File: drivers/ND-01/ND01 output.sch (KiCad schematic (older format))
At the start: 13 parts, among them J10 CONN_01X08, J11 CONN_01X08, J12 CONN_01X08, J13 CONN_01X08, J14 CONN_01X08, J15 CONN_01X08, J16 CONN_01X08, J4 CONN_01X08, J5 CONN_01X08, J6 CONN_01X08, J7 CONN_01X08, J8 CONN_01X08, J9 CONN_01X08

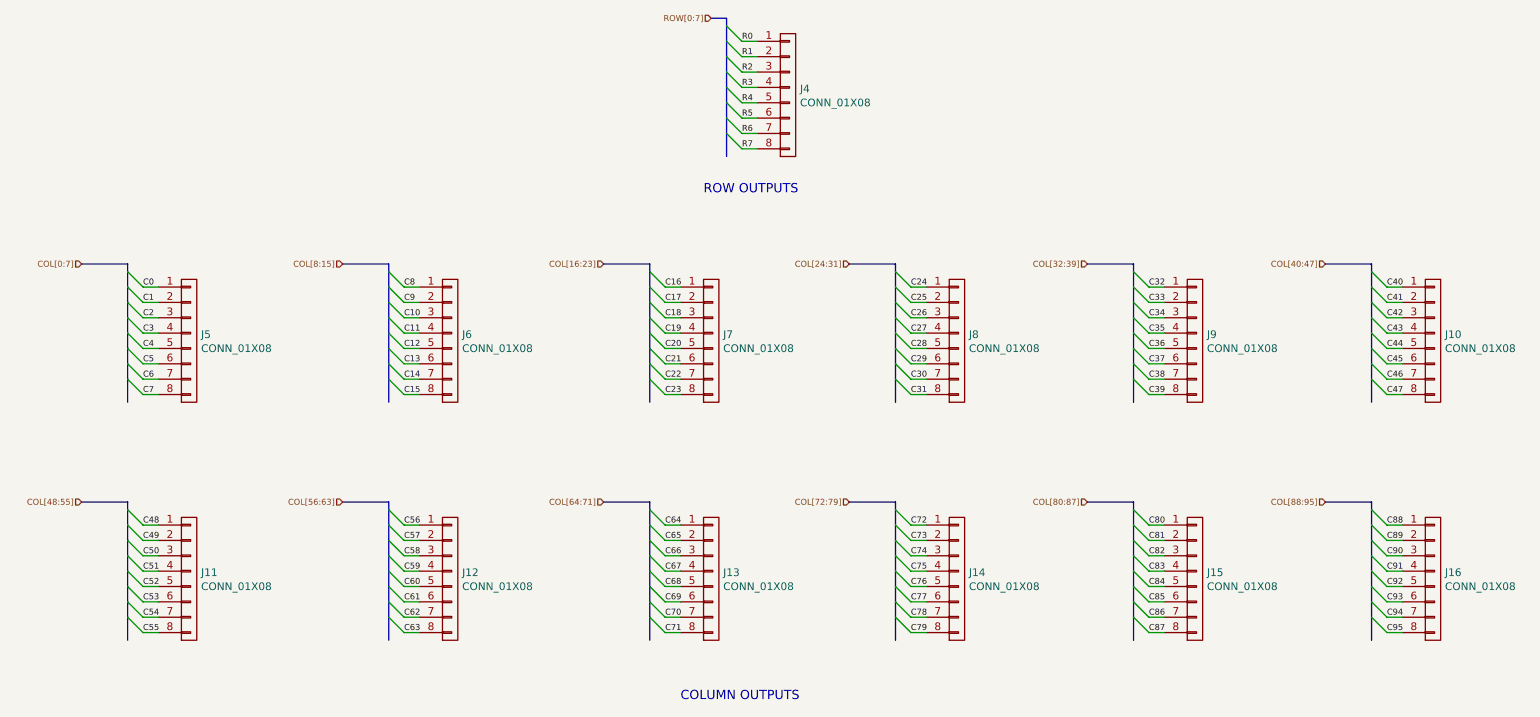
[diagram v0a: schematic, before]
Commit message: Add 2088xS LED dot matrix documentation pictures
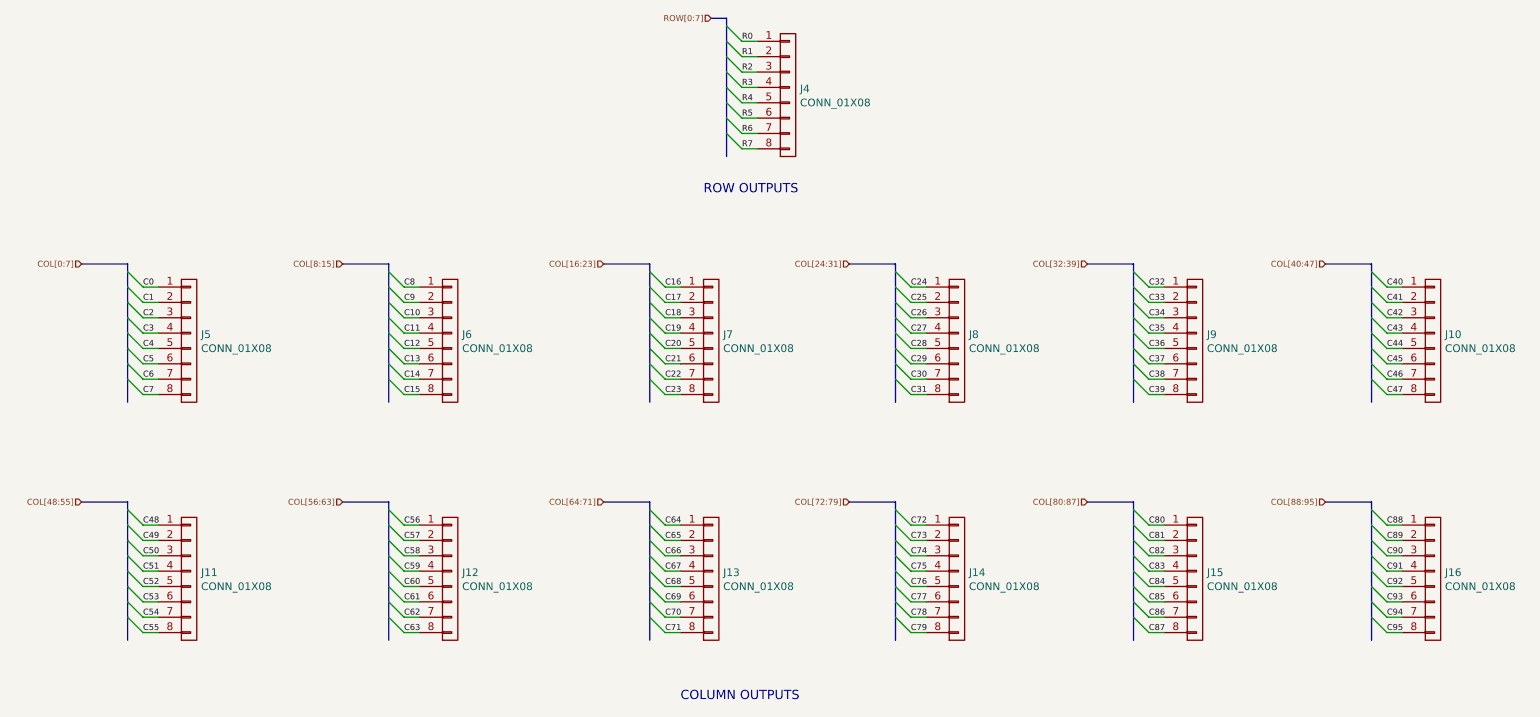
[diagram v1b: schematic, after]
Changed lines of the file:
@@
 	5300 900  5400 900
 Wire Bus Line
-	5400 900  5400 950
-Wire Bus Line
-	5400 950  5400 1050
-Wire Bus Line
-	5400 1050 5400 1150
-Wire Bus Line
-	5400 1150 5400 1250
-Wire Bus Line
-	5400 1250 5400 1350
-Wire Bus Line
-	5400 1350 5400 1450
-Wire Bus Line
-	5400 1450 5400 1550
-Wire Bus Line
-	5400 1550 5400 1650
-Wire Bus Line
-	5400 1650 5400 1800
+	5400 900  5400 1800
 $Comp
 L CONN_01X08 J4
@@
 	1200 2500 1500 2500
 Wire Bus Line
-	1500 2500 1500 2550
-Wire Bus Line
-	1500 2550 1500 2650
-Wire Bus Line
-	1500 2650 1500 2750
-Wire Bus Line
-	1500 2750 1500 2850
-Wire Bus Line
-	1500 2850 1500 2950
-Wire Bus Line
-	1500 2950 1500 3050
-Wire Bus Line
-	1500 3050 1500 3150
-Wire Bus Line
-	1500 3150 1500 3250
-Wire Bus Line
-	1500 3250 1500 3400
+	1500 2500 1500 3400
 $Comp
 L CONN_01X08 J5
@@
 	2900 2500 3200 2500
 Wire Bus Line
-	3200 2500 3200 2550
-Wire Bus Line
-	3200 2550 3200 2650
-Wire Bus Line
-	3200 2650 3200 2750
-Wire Bus Line
-	3200 2750 3200 2850
-Wire Bus Line
-	3200 2850 3200 2950
-Wire Bus Line
-	3200 2950 3200 3050
-Wire Bus Line
-	3200 3050 3200 3150
-Wire Bus Line
-	3200 3150 3200 3250
-Wire Bus Line
-	3200 3250 3200 3400
+	3200 2500 3200 3400
 $Comp
 L CONN_01X08 J6
@@
 	4600 2500 4900 2500
 Wire Bus Line
-	4900 2500 4900 2550
-Wire Bus Line
-	4900 2550 4900 2650
-Wire Bus Line
-	4900 2650 4900 2750
-Wire Bus Line
-	4900 2750 4900 2850
-Wire Bus Line
-	4900 2850 4900 2950
-Wire Bus Line
-	4900 2950 4900 3050
-Wire Bus Line
-	4900 3050 4900 3150
-Wire Bus Line
-	4900 3150 4900 3250
-Wire Bus Line
-	4900 3250 4900 3400
+	4900 2500 4900 3400
 $Comp
 L CONN_01X08 J7
@@
 	6200 2500 6500 2500
 Wire Bus Line
-	6500 2500 6500 2550
-Wire Bus Line
-	6500 2550 6500 2650
-Wire Bus Line
-	6500 2650 6500 2750
-Wire Bus Line
-	6500 2750 6500 2850
-Wire Bus Line
-	6500 2850 6500 2950
-Wire Bus Line
-	6500 2950 6500 3050
-Wire Bus Line
-	6500 3050 6500 3150
-Wire Bus Line
-	6500 3150 6500 3250
-Wire Bus Line
-	6500 3250 6500 3400
+	6500 2500 6500 3400
 $Comp
 L CONN_01X08 J8
@@
 	7750 2500 8050 2500
 Wire Bus Line
-	8050 2500 8050 2550
-Wire Bus Line
-	8050 2550 8050 2650
-Wire Bus Line
-	8050 2650 8050 2750
-Wire Bus Line
-	8050 2750 8050 2850
-Wire Bus Line
-	8050 2850 8050 2950
-Wire Bus Line
-	8050 2950 8050 3050
-Wire Bus Line
-	8050 3050 8050 3150
-Wire Bus Line
-	8050 3150 8050 3250
-Wire Bus Line
-	8050 3250 8050 3400
+	8050 2500 8050 3400
 $Comp
 L CONN_01X08 J9
@@
 	9300 2500 9600 2500
 Wire Bus Line
-	9600 2500 9600 2550
-Wire Bus Line
-	9600 2550 9600 2650
-Wire Bus Line
-	9600 2650 9600 2750
-Wire Bus Line
-	9600 2750 9600 2850
-Wire Bus Line
-	9600 2850 9600 2950
-Wire Bus Line
-	9600 2950 9600 3050
-Wire Bus Line
-	9600 3050 9600 3150
-Wire Bus Line
-	9600 3150 9600 3250
-Wire Bus Line
-	9600 3250 9600 3400
+	9600 2500 9600 3400
 $Comp
 L CONN_01X08 J10
@@
 	1200 4050 1500 4050
 Wire Bus Line
-	1500 4050 1500 4100
-Wire Bus Line
-	1500 4100 1500 4200
-Wire Bus Line
-	1500 4200 1500 4300
-Wire Bus Line
-	1500 4300 1500 4400
-Wire Bus Line
-	1500 4400 1500 4500
-Wire Bus Line
-	1500 4500 1500 4600
-Wire Bus Line
-	1500 4600 1500 4700
-Wire Bus Line
-	1500 4700 1500 4800
-Wire Bus Line
-	1500 4800 1500 4950
+	1500 4050 1500 4950
 $Comp
 L CONN_01X08 J11
@@
 	2900 4050 3200 4050
 Wire Bus Line
-	3200 4050 3200 4100
-Wire Bus Line
-	3200 4100 3200 4200
-Wire Bus Line
-	3200 4200 3200 4300
-Wire Bus Line
-	3200 4300 3200 4400
-Wire Bus Line
-	3200 4400 3200 4500
-Wire Bus Line
-	3200 4500 3200 4600
-Wire Bus Line
-	3200 4600 3200 4700
-Wire Bus Line
-	3200 4700 3200 4800
-Wire Bus Line
-	3200 4800 3200 4950
+	3200 4050 3200 4950
 $Comp
 L CONN_01X08 J12
@@
 	4600 4050 4900 4050
 Wire Bus Line
-	4900 4050 4900 4100
-Wire Bus Line
-	4900 4100 4900 4200
-Wire Bus Line
-	4900 4200 4900 4300
-Wire Bus Line
-	4900 4300 4900 4400
-Wire Bus Line
-	4900 4400 4900 4500
-Wire Bus Line
-	4900 4500 4900 4600
-Wire Bus Line
-	4900 4600 4900 4700
-Wire Bus Line
-	4900 4700 4900 4800
-Wire Bus Line
-	4900 4800 4900 4950
+	4900 4050 4900 4950
 $Comp
 L CONN_01X08 J13
@@
 	6200 4050 6500 4050
 Wire Bus Line
-	6500 4050 6500 4100
-Wire Bus Line
-	6500 4100 6500 4200
-Wire Bus Line
-	6500 4200 6500 4300
-Wire Bus Line
-	6500 4300 6500 4400
-Wire Bus Line
-	6500 4400 6500 4500
-Wire Bus Line
-	6500 4500 6500 4600
-Wire Bus Line
-	6500 4600 6500 4700
-Wire Bus Line
-	6500 4700 6500 4800
-Wire Bus Line
-	6500 4800 6500 4950
+	6500 4050 6500 4950
 $Comp
 L CONN_01X08 J14
@@
 	7750 4050 8050 4050
 Wire Bus Line
-	8050 4050 8050 4100
-Wire Bus Line
-	8050 4100 8050 4200
-Wire Bus Line
-	8050 4200 8050 4300
-Wire Bus Line
-	8050 4300 8050 4400
-Wire Bus Line
-	8050 4400 8050 4500
-Wire Bus Line
-	8050 4500 8050 4600
-Wire Bus Line
-	8050 4600 8050 4700
-Wire Bus Line
-	8050 4700 8050 4800
-Wire Bus Line
-	8050 4800 8050 4950
+	8050 4050 8050 4950
 $Comp
 L CONN_01X08 J15
@@
 	9300 4050 9600 4050
 Wire Bus Line
-	9600 4050 9600 4100
-Wire Bus Line
-	9600 4100 9600 4200
-Wire Bus Line
-	9600 4200 9600 4300
-Wire Bus Line
-	9600 4300 9600 4400
-Wire Bus Line
-	9600 4400 9600 4500
-Wire Bus Line
-	9600 4500 9600 4600
-Wire Bus Line
-	9600 4600 9600 4700
-Wire Bus Line
-	9600 4700 9600 4800
-Wire Bus Line
-	9600 4800 9600 4950
+	9600 4050 9600 4950
 $Comp
 L CONN_01X08 J16
